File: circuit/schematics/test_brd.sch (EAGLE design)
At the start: 5 parts

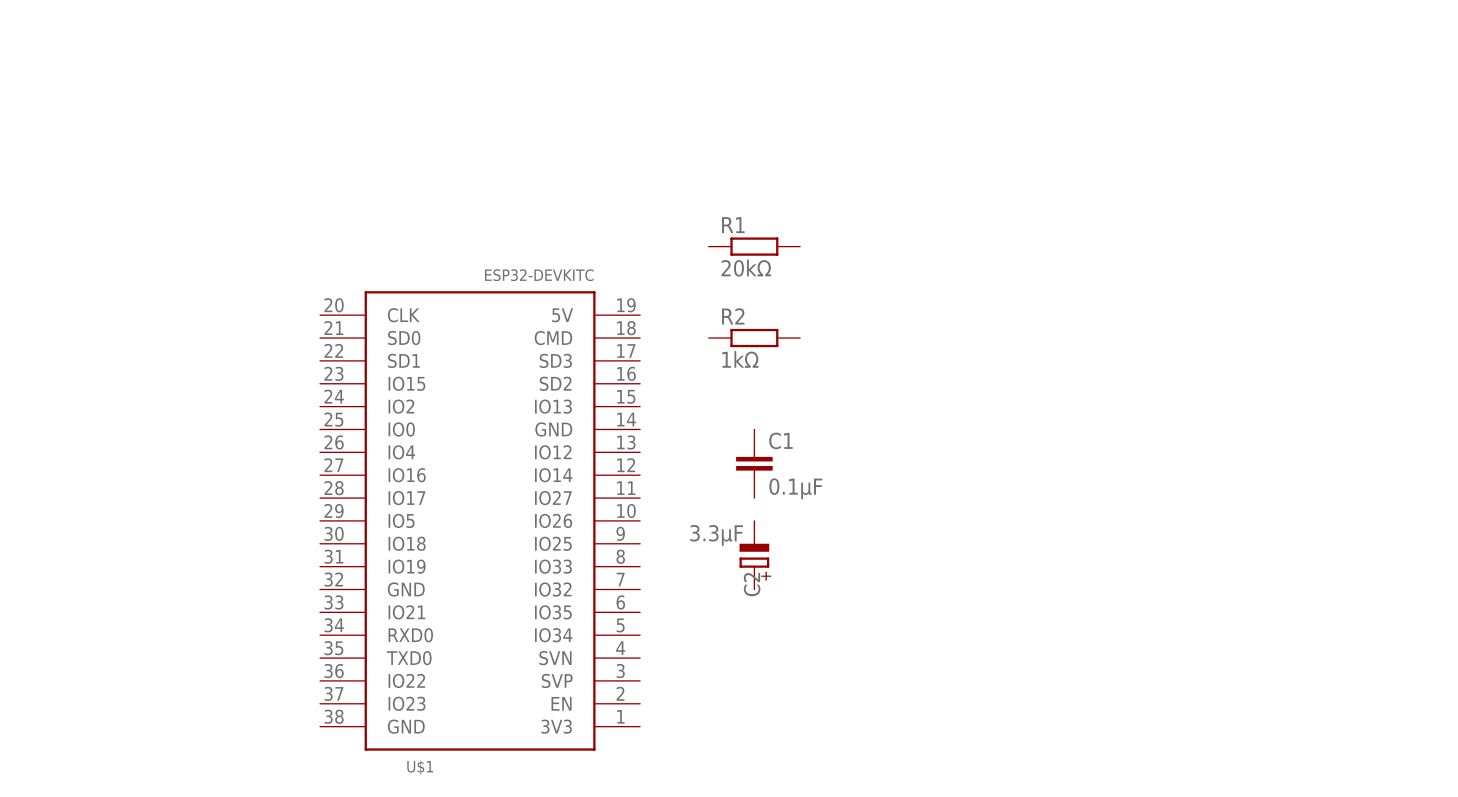
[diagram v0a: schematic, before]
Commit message: dekita
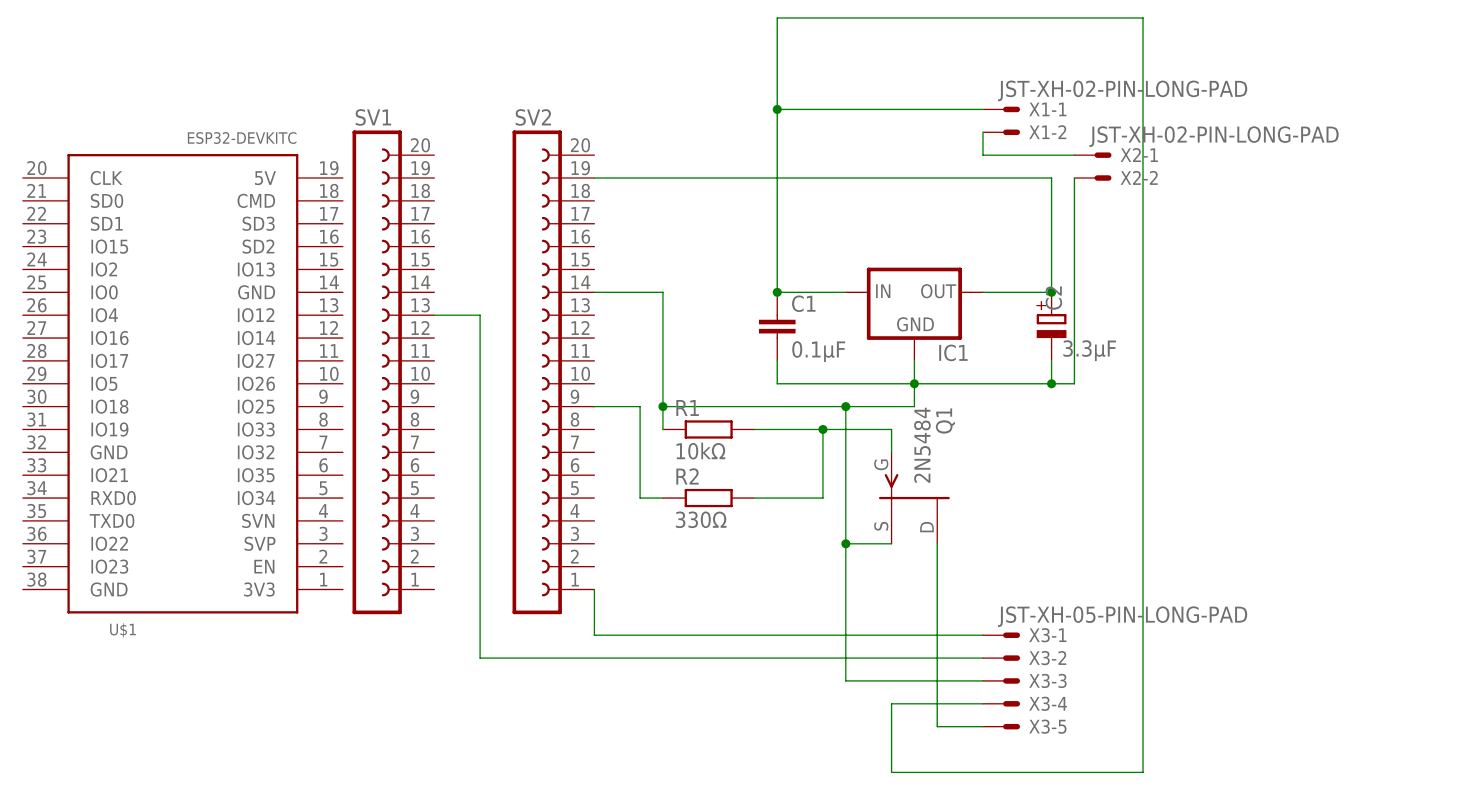
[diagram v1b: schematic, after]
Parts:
- added IC1: (no value), v-reg:78XXS
- added Q1: 2N5484, transistor-fet:2N5484
- added SV1, SV2: (no value), con-lsta:FE20-1
- added X1, X2: JST-XH-02-PIN-LONG-PAD, Rembrandt Electronics - JST XH Connectors v1-0:JST-XH-02-PIN-LONG-PAD
- added X3: JST-XH-05-PIN-LONG-PAD, Rembrandt Electronics - JST XH Connectors v1-0:JST-XH-05-PIN-LONG-PAD
- R1: value 20kΩ -> 10kΩ
- R2: value 1kΩ -> 330Ω
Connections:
- new net N$1: C1.1, IC1.IN, X1-1.S, X3-4.S
- new net N$2: C2.+, IC1.OUT, SV2.19
- new net N$3: C1.2, C2.-, IC1.GND, Q1.S, R1.1, SV2.14, X2-2.S, X3-3.S
- new net N$4: Q1.G, R1.2, R2.2
- new net N$5: R2.1, SV2.9
- new net N$6: X1-2.S, X2-1.S
- new net N$7: SV2.1, X3-1.S
- new net N$8: SV1.13, X3-2.S
- new net N$9: Q1.D, X3-5.S
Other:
- moved on the sheet: C1, C2, R1, R2, U$1
